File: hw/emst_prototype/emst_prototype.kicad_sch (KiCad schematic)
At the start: 35 parts, among them J1 USB_B_Micro, U1 AD5940BCBZ-RL, Y1 ABM8-16.000MHZ-B2-T

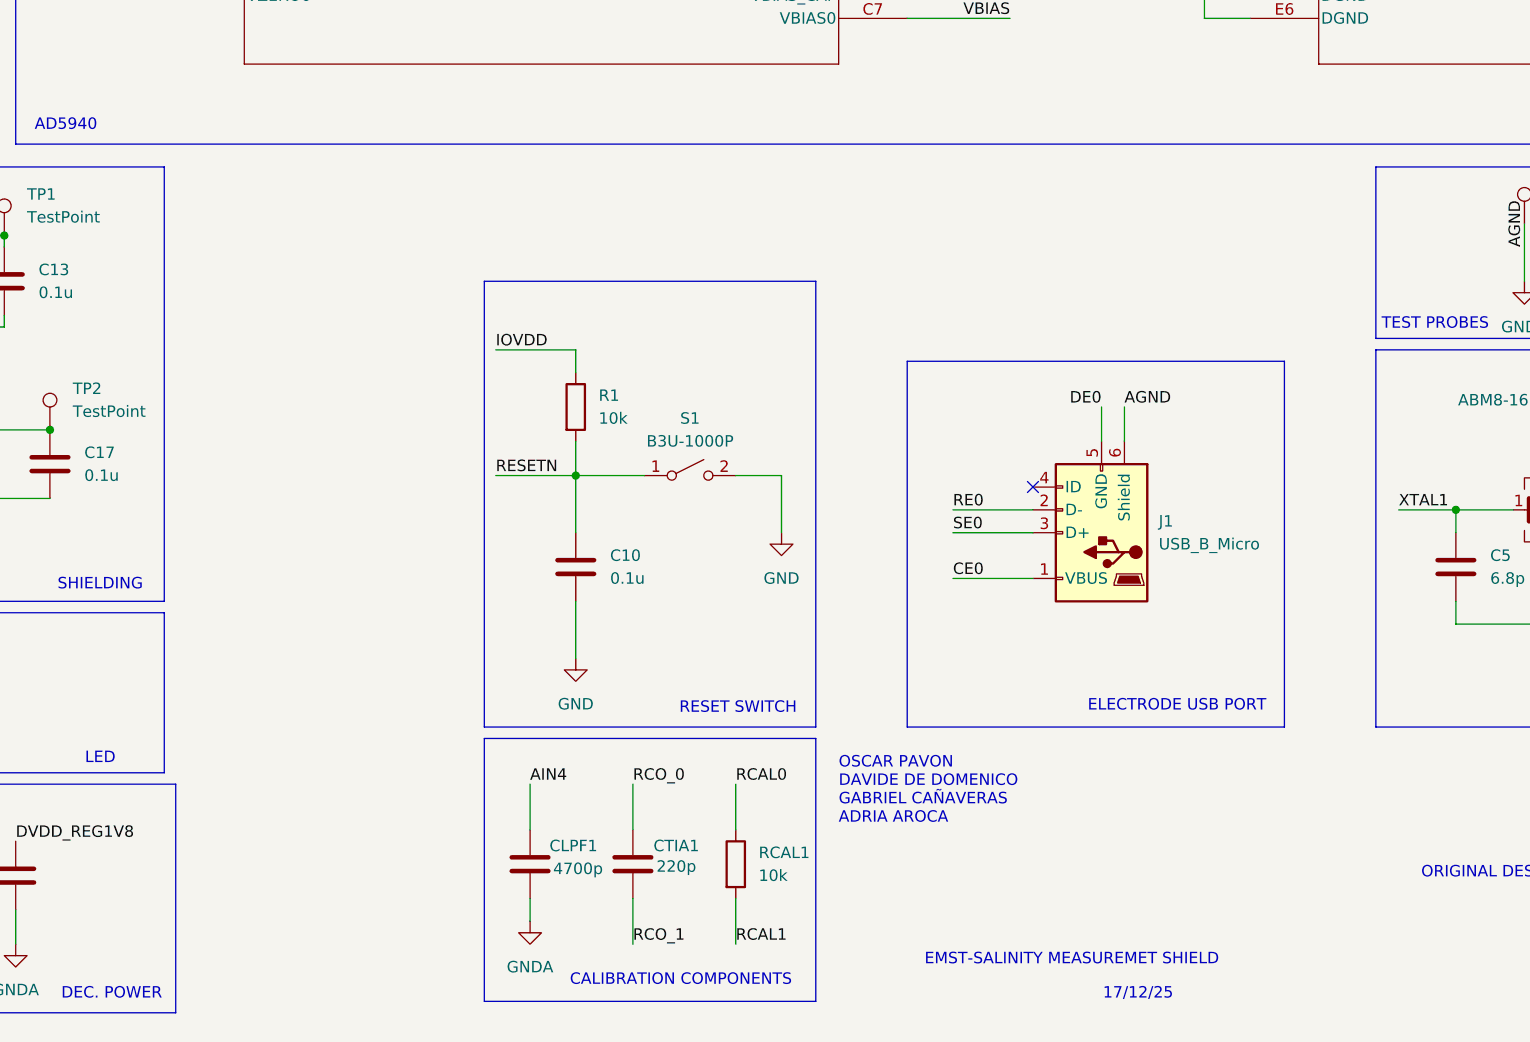
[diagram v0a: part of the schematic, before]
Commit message: Added Voltage Regulator
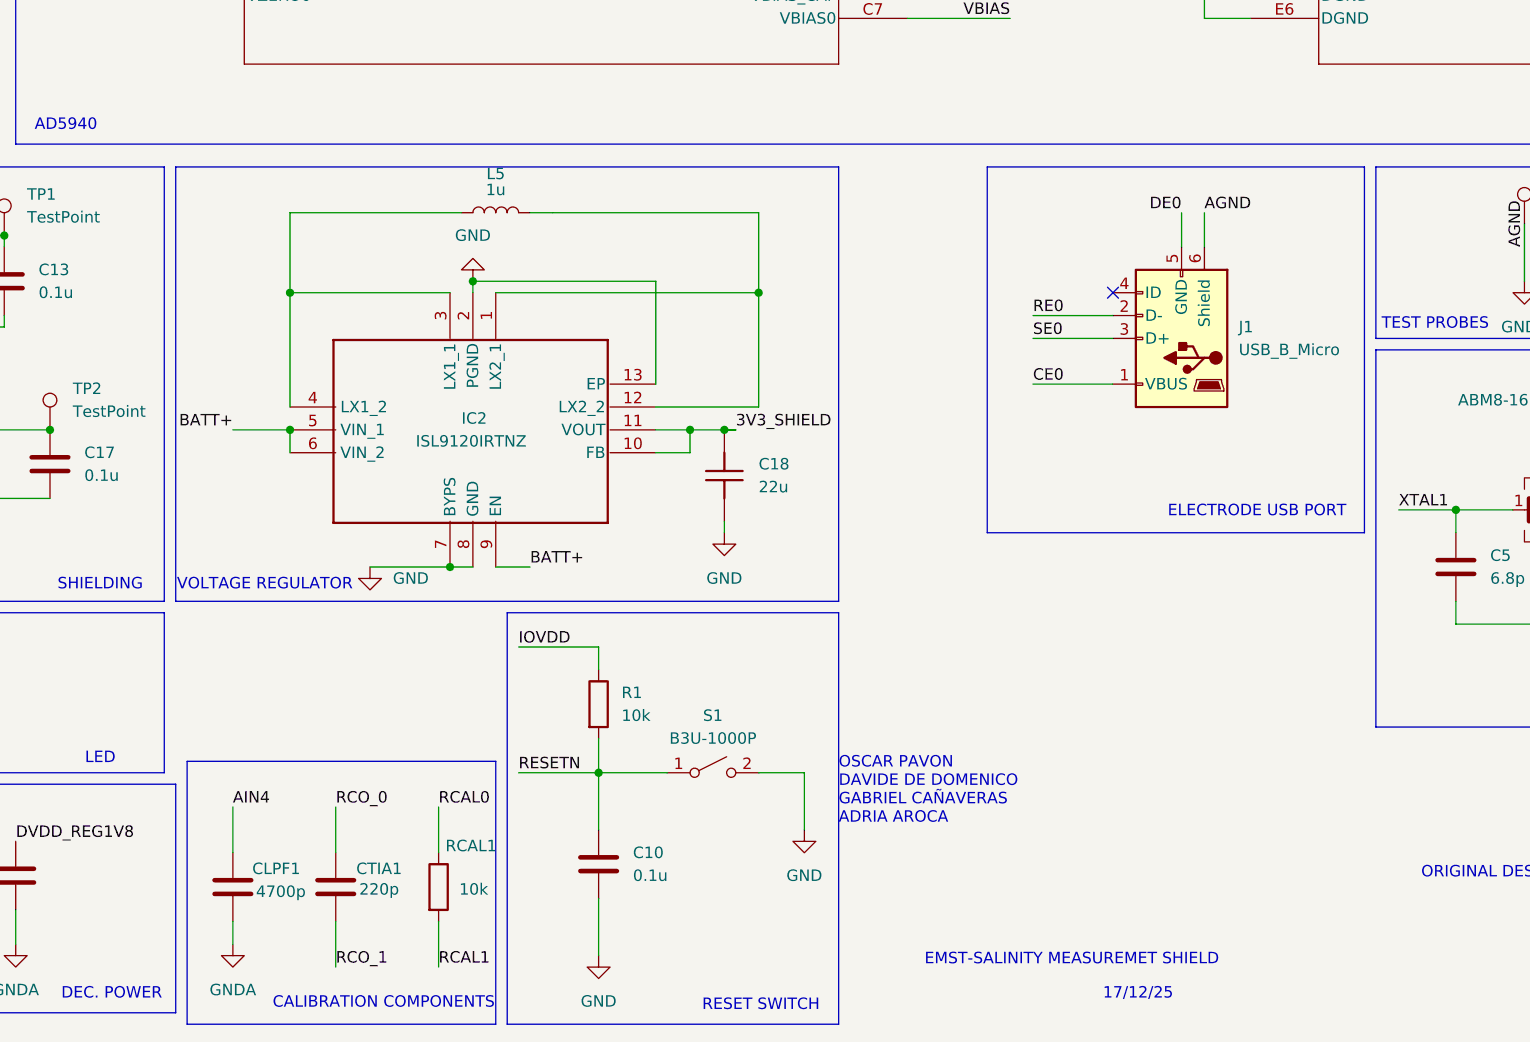
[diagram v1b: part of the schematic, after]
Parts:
- added C18: 22u, Capacitor_SMD:C_0603_1608Metric, symbol PCB-EPS-altium-import:1_22u
- added IC2: ISL9120IRTNZ, power-nsl:ISL9120IRTNZ, symbol -nsl_power:ISL9120IRTNZ
- added L5: 1u, Inductor_SMD:L_0805_2012Metric, symbol Device:L
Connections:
- net 3V3_SHIELD: now also C18.2, IC2.10 (FB), IC2.11 (VOUT)
- net GND: now also C18.1, IC2.13 (EP), IC2.2 (PGND), IC2.7 (BYPS), IC2.8 (GND)
- new net: IC2.1 (LX2_1), IC2.12 (LX2_2), L5.2
- new net: IC2.3 (LX1_1), IC2.4 (LX1_2), L5.1
- new net BATT+: IC2.5 (VIN_1), IC2.6 (VIN_2), IC2.9 (EN)
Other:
- note added: "VOLTAGE REGULATOR"
- moved on the sheet: C10, CLPF1, CTIA1, J1, R1, RCAL1, S1
